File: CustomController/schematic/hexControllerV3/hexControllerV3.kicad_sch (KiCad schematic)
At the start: 48 parts, among them IC1 ESP32-S2-MINI-1-N4R2, IC2 IP5306, J1 USB_C_Receptacle_USB2.0_16P, J2 Battery, J3 Switch1, J4 Switch2, J5 Switch3, J6 Switch4, J7 Battery, SW1 RotaryEncoder_Switch, SW2 SW_DIP_x01, SW3 SW_DIP_x01, SW4 SW_DIP_x01, SW5 SW_DIP_x01, SW6 SW_DIP_x01, U2 AMS1117-3.3

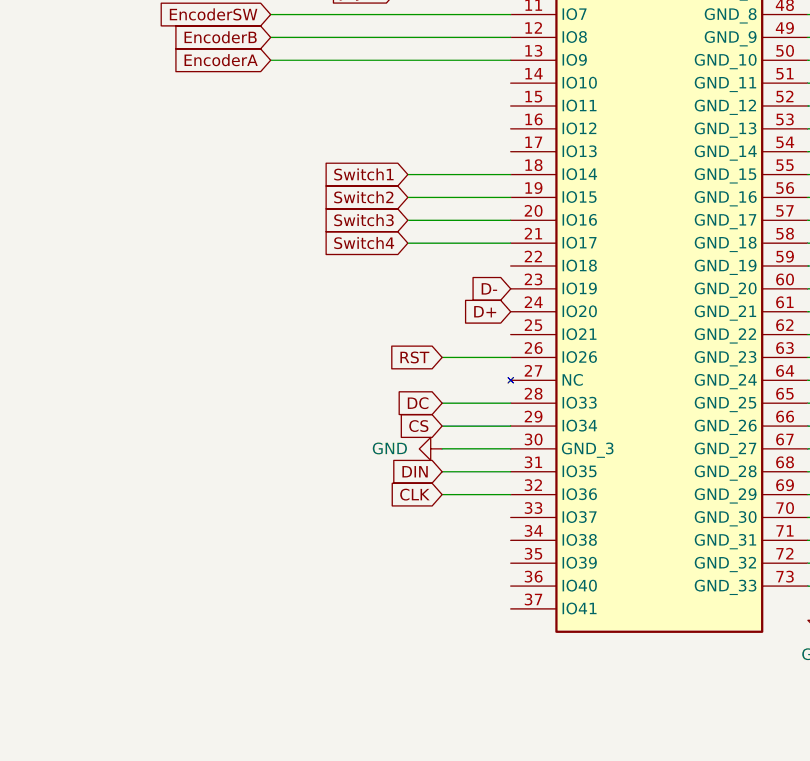
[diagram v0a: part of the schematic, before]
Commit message: Improved PCB design
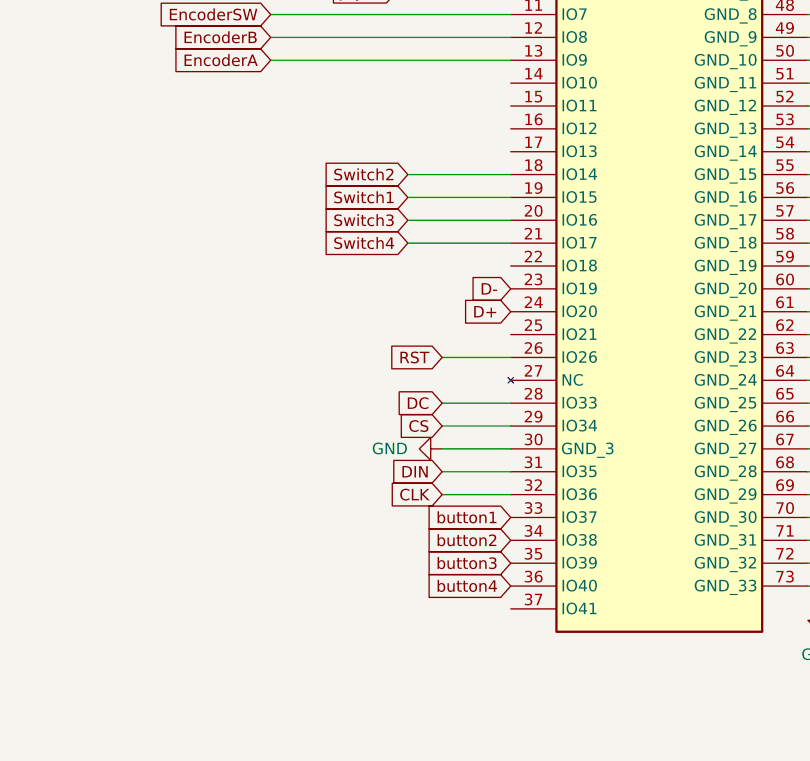
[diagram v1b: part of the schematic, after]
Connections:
- net Switch1: now also IC1.19 (IO15); no longer IC1.18 (IO14)
- net Switch2: now also IC1.18 (IO14); no longer IC1.19 (IO15)
- net button1: now also IC1.33 (IO37)
- net button2: now also IC1.34 (IO38)
- net button3: now also IC1.35 (IO39)
- net button4: now also IC1.36 (IO40)
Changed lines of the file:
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@@
+		)
+	)
+	(global_label "button4"
+		(shape input)
+		(at 184.15 115.57 180)
+		(fields_autoplaced yes)
+		(effects
+			(font
+				(size 1.27 1.27)
+			)
+			(justify right)
+		)
+		(property "Intersheetrefs" "${INTERSHEET_REFS}"
+			(at 173.9079 115.57 0)
+			(effects
+				(font
+					(size 1.27 1.27)
+				)
+				(justify right)
+				(hide yes)
+			)
 		)
 	)
@@
 		)
 	)
+	(global_label "button2"
+		(shape input)
+		(at 184.15 110.49 180)
+		(fields_autoplaced yes)
+		(effects
+			(font
+				(size 1.27 1.27)
+			)
+			(justify right)
+		)
+		(property "Intersheetrefs" "${INTERSHEET_REFS}"
+			(at 173.9079 110.49 0)
+			(effects
+				(font
+					(size 1.27 1.27)
+				)
+				(justify right)
+				(hide yes)
+			)
+		)
+	)
 	(global_label "Switch3"
 		(shape input)
@@
 		)
 	)
+	(global_label "button3"
+		(shape input)
+		(at 184.15 113.03 180)
+		(fields_autoplaced yes)
+		(effects
+			(font
+				(size 1.27 1.27)
+			)
+			(justify right)
+		)
+		(property "Intersheetrefs" "${INTERSHEET_REFS}"
+			(at 173.9079 113.03 0)
+			(effects
+				(font
+					(size 1.27 1.27)
+				)
+				(justify right)
+				(hide yes)
+			)
+		)
+	)
 	(global_label "DIN"
 		(shape input)
@@
 		)
 	)
+	(global_label "button1"
+		(shape input)
+		(at 184.15 107.95 180)
+		(fields_autoplaced yes)
+		(effects
+			(font
+				(size 1.27 1.27)
+			)
+			(justify right)
+		)
+		(property "Intersheetrefs" "${INTERSHEET_REFS}"
+			(at 173.9079 107.95 0)
+			(effects
+				(font
+					(size 1.27 1.27)
+				)
+				(justify right)
+				(hide yes)
+			)
+		)
+	)
 	(global_label "D-"
 		(shape input)
@@
 	(global_label "Switch2"
 		(shape input)
+		(at 172.72 69.85 180)
+		(fields_autoplaced yes)
+		(effects
+			(font
+				(size 1.27 1.27)
+			)
+			(justify right)
+		)
+		(property "Intersheetrefs" "${INTERSHEET_REFS}"
+			(at 162.4172 69.85 0)
+			(effects
+				(font
+					(size 1.27 1.27)
+				)
+				(justify right)
+				(hide yes)
+			)
+		)
+	)
+	(global_label "EncoderSW"
+		(shape input)
+		(at 157.48 52.07 180)
+		(fields_autoplaced yes)
+		(effects
+			(font
+				(size 1.27 1.27)
+			)
+			(justify right)
+		)
+		(property "Intersheetrefs" "${INTERSHEET_REFS}"
+			(at 145.8468 52.07 0)
+			(effects
+				(font
+					(size 1.27 1.27)
+				)
+				(justify right)
+				(hide yes)
+			)
+		)
+	)
+	(global_label "BOOT"
+		(shape input)
+		(at 184.15 34.29 180)
+		(fields_autoplaced yes)
+		(effects
+			(font
+				(size 1.27 1.27)
+			)
+			(justify right)
+		)
+		(property "Intersheetrefs" "${INTERSHEET_REFS}"
+			(at 176.2662 34.29 0)
+			(effects
+				(font
+					(size 1.27 1.27)
+				)
+				(justify right)
+				(hide yes)
+			)
+		)
+	)
+	(global_label "Joy1Y"
+		(shape input)
+		(at 158.75 36.83 180)
+		(fields_autoplaced yes)
+		(effects
+			(font
+				(size 1.27 1.27)
+			)
+			(justify right)
+		)
+		(property "Intersheetrefs" "${INTERSHEET_REFS}"
+			(at 150.2616 36.83 0)
+			(effects
+				(font
+					(size 1.27 1.27)
+				)
+				(justify right)
+				(hide yes)
+			)
+		)
+	)
+	(global_label "Joy1X"
+		(shape input)
+		(at 158.75 39.37 180)
+		(fields_autoplaced yes)
+		(effects
+			(font
+				(size 1.27 1.27)
+			)
+			(justify right)
+		)
+		(property "Intersheetrefs" "${INTERSHEET_REFS}"
+			(at 150.3825 39.37 0)
+			(effects
+				(font
+					(size 1.27 1.27)
+				)
+				(justify right)
+				(hide yes)
+			)
+		)
+	)
+	(global_label "EN"
+		(shape input)
+		(at 59.69 256.54 180)
+		(fields_autoplaced yes)
+		(effects
+			(font
+				(size 1.27 1.27)
+			)
+			(justify right)
+		)
+		(property "Intersheetrefs" "${INTERSHEET_REFS}"
+			(at 54.2253 256.54 0)
+			(effects
+				(font
+					(size 1.27 1.27)
+				)
+				(justify right)
+				(hide yes)
+			)
+		)
+	)
+	(global_label "DC"
+		(shape input)
+		(at 29.21 22.86 0)
+		(fields_autoplaced yes)
+		(effects
+			(font
+				(size 1.27 1.27)
+			)
+			(justify left)
+		)
+		(property "Intersheetrefs" "${INTERSHEET_REFS}"
+			(at 34.7352 22.86 0)
+			(effects
+				(font
+					(size 1.27 1.27)
+				)
+				(justify left)
+				(hide yes)
+			)
+		)
+	)
+	(global_label "Joy2Y"
+		(shape input)
+		(at 24.13 86.36 180)
+		(fields_autoplaced yes)
+		(effects
+			(font
+				(size 1.27 1.27)
+			)
+			(justify right)
+		)
+		(property "Intersheetrefs" "${INTERSHEET_REFS}"
+			(at 15.7625 86.36 0)
+			(effects
+				(font
+					(size 1.27 1.27)
+				)
+				(justify right)
+				(hide yes)
+			)
+		)
+	)
+	(global_label "Switch1"
+		(shape input)
 		(at 172.72 72.39 180)
 		(fields_autoplaced yes)
@@
 			(effects
 				(font
-					(size 1.27 1.27)
-				)
-				(justify right)
-				(hide yes)
-			)
-		)
-	)
-	(global_label "EncoderSW"
-		(shape input)
-		(at 157.48 52.07 180)
-		(fields_autoplaced yes)
-		(effects
-			(font
-				(size 1.27 1.27)
-			)
-			(justify right)
-		)
-		(property "Intersheetrefs" "${INTERSHEET_REFS}"
-			(at 145.8468 52.07 0)
-			(effects
-				(font
-					(size 1.27 1.27)
-				)
-				(justify right)
-				(hide yes)
-			)
-		)
-	)
-	(global_label "BOOT"
-		(shape input)
-		(at 184.15 34.29 180)
-		(fields_autoplaced yes)
-		(effects
-			(font
-				(size 1.27 1.27)
-			)
-			(justify right)
-		)
-		(property "Intersheetrefs" "${INTERSHEET_REFS}"
-			(at 176.2662 34.29 0)
-			(effects
-				(font
-					(size 1.27 1.27)
-				)
-				(justify right)
-				(hide yes)
-			)
-		)
-	)
-	(global_label "Joy1Y"
-		(shape input)
-		(at 158.75 36.83 180)
-		(fields_autoplaced yes)
-		(effects
-			(font
-				(size 1.27 1.27)
-			)
-			(justify right)
-		)
-		(property "Intersheetrefs" "${INTERSHEET_REFS}"
-			(at 150.2616 36.83 0)
-			(effects
-				(font
-					(size 1.27 1.27)
-				)
-				(justify right)
-				(hide yes)
-			)
-		)
-	)
-	(global_label "Joy1X"
-		(shape input)
-		(at 158.75 39.37 180)
-		(fields_autoplaced yes)
-		(effects
-			(font
-				(size 1.27 1.27)
-			)
-			(justify right)
-		)
-		(property "Intersheetrefs" "${INTERSHEET_REFS}"
-			(at 150.3825 39.37 0)
-			(effects
-				(font
-					(size 1.27 1.27)
-				)
-				(justify right)
-				(hide yes)
-			)
-		)
-	)
-	(global_label "EN"
-		(shape input)
-		(at 59.69 256.54 180)
-		(fields_autoplaced yes)
-		(effects
-			(font
-				(size 1.27 1.27)
-			)
-			(justify right)
-		)
-		(property "Intersheetrefs" "${INTERSHEET_REFS}"
-			(at 54.2253 256.54 0)
-			(effects
-				(font
-					(size 1.27 1.27)
-				)
-				(justify right)
-				(hide yes)
-			)
-		)
-	)
-	(global_label "DC"
-		(shape input)
-		(at 29.21 22.86 0)
-		(fields_autoplaced yes)
-		(effects
-			(font
-				(size 1.27 1.27)
-			)
-			(justify left)
-		)
-		(property "Intersheetrefs" "${INTERSHEET_REFS}"
-			(at 34.7352 22.86 0)
-			(effects
-				(font
-					(size 1.27 1.27)
-				)
-				(justify left)
-				(hide yes)
-			)
-		)
-	)
-	(global_label "Joy2Y"
-		(shape input)
-		(at 24.13 86.36 180)
-		(fields_autoplaced yes)
-		(effects
-			(font
-				(size 1.27 1.27)
-			)
-			(justify right)
-		)
-		(property "Intersheetrefs" "${INTERSHEET_REFS}"
-			(at 15.7625 86.36 0)
-			(effects
-				(font
-					(size 1.27 1.27)
-				)
-				(justify right)
-				(hide yes)
-			)
-		)
-	)
-	(global_label "Switch1"
-		(shape input)
-		(at 172.72 69.85 180)
-		(fields_autoplaced yes)
-		(effects
-			(font
-				(size 1.27 1.27)
-			)
-			(justify right)
-		)
-		(property "Intersheetrefs" "${INTERSHEET_REFS}"
-			(at 162.4172 69.85 0)
-			(effects
-				(font
